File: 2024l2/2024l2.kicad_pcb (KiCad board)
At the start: 2 copper layers, 174 x 141 mm, 113 parts, among them IC1 LM2587S-ADJ, IC2 VNH5019ATR-E, IC3 VNH5019ATR-E, IC4 VNH5019ATR-E, IC5 VNH5019ATR-E, J1 Conn_01x02, J2 Conn_01x02, J3 Conn_01x03, J4 Conn_01x03, J5 Conn_01x04, J6 Conn_01x06, Q1 AON6354, Q2 AON6354, Q3 AON6354, Q4 AON6354, SW1 SW_SPDT, U1 TPS5430DDA, U2 TPS5430DDA, U3 Teensy 4.0

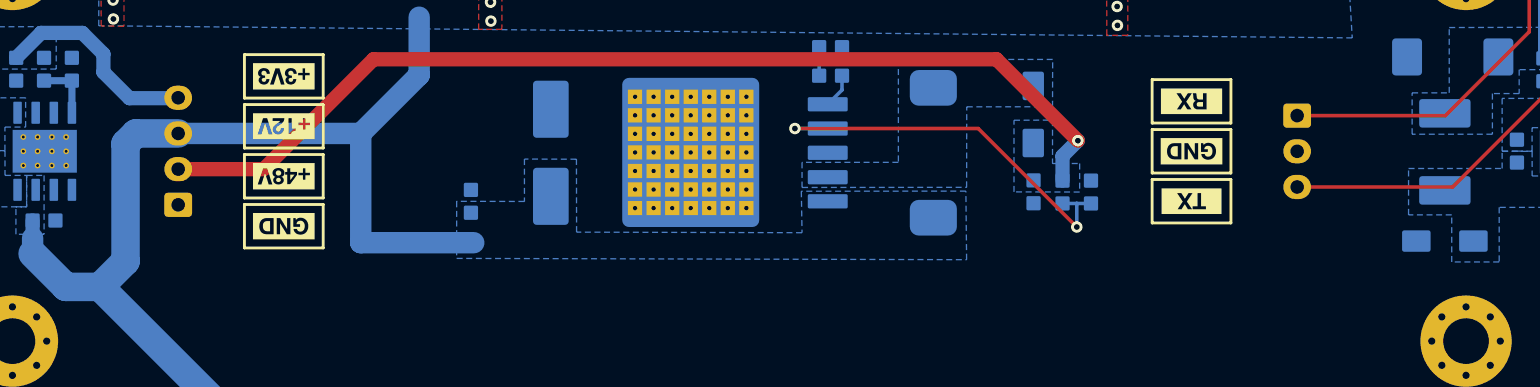
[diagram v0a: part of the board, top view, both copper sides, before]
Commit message: Minor trace adjustment
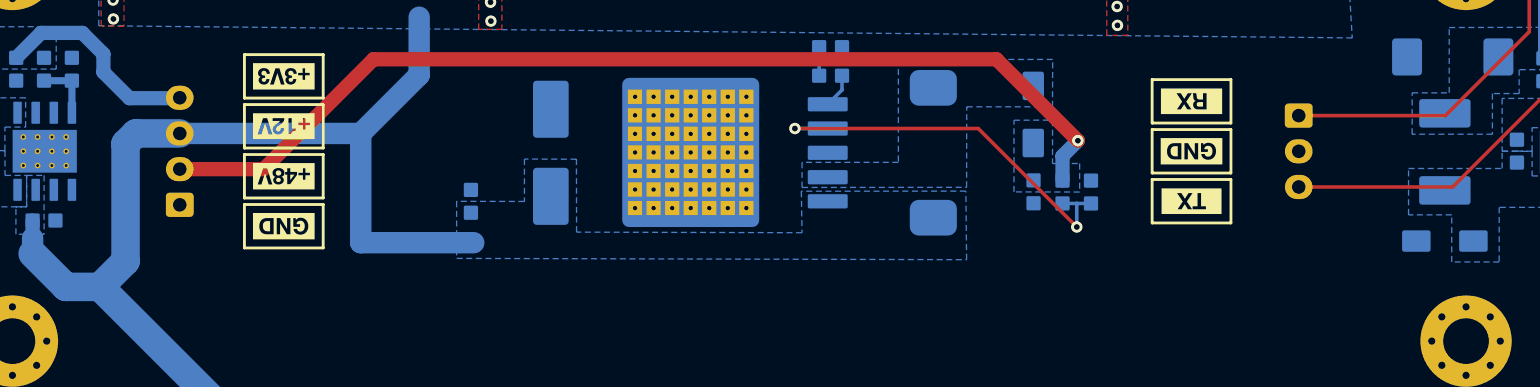
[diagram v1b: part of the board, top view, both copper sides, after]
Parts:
- moved J5 0.11 mm to (109.3, 213.6)
- moved J3 0.11 mm to (187.7, 207.4)
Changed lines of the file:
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@@
   )
   (footprint "Connector_JST:JST_XH_B4B-XH-A_1x04_P2.50mm_Vertical" (layer "B.Cu")
-    (at 109.18985 213.645 90)
+    (at 109.3 213.645 90)
     (descr "JST XH series connector, B4B-XH-A (http://www.jst-mfg.com/product/pdf/eng/eXH.pdf), generated with kicad-footprint-generator")
     (tags "connector JST XH vertical")
@@
   )
   (footprint "Connector_JST:JST_XH_B3B-XH-A_1x03_P2.50mm_Vertical" (layer "B.Cu")
-    (at 187.58985 207.395 -90)
+    (at 187.7 207.395 -90)
     (descr "JST XH series connector, B3B-XH-A (http://www.jst-mfg.com/product/pdf/eng/eXH.pdf), generated with kicad-footprint-generator")
     (tags "connector JST XH vertical")
@@
   (segment (start 124.125 151.975) (end 124.125 156.75) (width 1) (layer "F.Cu") (net 4))
   (via (at 124.125 151.975) (size 0.8) (drill 0.4) (layers "F.Cu" "B.Cu") (net 4))
+  (segment (start 99.58485 201.6) (end 102.475 201.6) (width 1) (layer "B.Cu") (net 4))
   (segment (start 124.125 139.3) (end 128.7 134.725) (width 1) (layer "B.Cu") (net 4))
+  (segment (start 92.8 183.3) (end 92.8 201.35515) (width 1) (layer "B.Cu") (net 4))
+  (segment (start 103.95 204.35) (end 105.775 206.175) (width 1) (layer "B.Cu") (net 4))
+  (segment (start 94.68985 203.245) (end 94.251637 202.806787) (width 0.25) (layer "B.Cu") (net 4))
+  (segment (start 124.125 151.975) (end 92.8 183.3) (width 1) (layer "B.Cu") (net 4))
+  (segment (start 103.95 203.075) (end 103.95 204.35) (width 1) (layer "B.Cu") (net 4))
+  (segment (start 144.6 132.025) (end 144.6 130.4) (width 1) (layer "B.Cu") (net 4))
+  (segment (start 105.775 206.175) (end 109.15985 206.175) (width 1) (layer "B.Cu") (net 4))
+  (segment (start 128.7 134.725) (end 141.9 134.725) (width 1) (layer "B.Cu") (net 4))
+  (segment (start 97.83985 203.345) (end 99.58485 201.6) (width 1) (layer "B.Cu") (net 4))
   (segment (start 102.475 201.6) (end 103.95 203.075) (width 1) (layer "B.Cu") (net 4))
-  (segment (start 103.95 203.075) (end 103.95 204.35) (width 1) (layer "B.Cu") (net 4))
-  (segment (start 105.775 206.175) (end 109.15985 206.175) (width 1) (layer "B.Cu") (net 4))
-  (segment (start 103.95 204.35) (end 105.775 206.175) (width 1) (layer "B.Cu") (net 4))
-  (segment (start 92.8 183.3) (end 92.8 201.35515) (width 1) (layer "B.Cu") (net 4))
-  (segment (start 94.68985 203.245) (end 94.251637 202.806787) (width 0.25) (layer "B.Cu") (net 4))
-  (segment (start 99.58485 201.6) (end 102.475 201.6) (width 1) (layer "B.Cu") (net 4))
-  (segment (start 97.83985 203.345) (end 99.58485 201.6) (width 1) (layer "B.Cu") (net 4))
+  (segment (start 124.125 151.975) (end 124.125 139.3) (width 1) (layer "B.Cu") (net 4))
   (segment (start 109.15985 206.175) (end 109.18985 206.145) (width 1) (layer "B.Cu") (net 4))
-  (segment (start 124.125 151.975) (end 92.8 183.3) (width 1) (layer "B.Cu") (net 4))
-  (segment (start 144.6 132.025) (end 144.6 130.4) (width 1) (layer "B.Cu") (net 4))
-  (segment (start 128.7 134.725) (end 141.9 134.725) (width 1) (layer "B.Cu") (net 4))
-  (segment (start 124.125 151.975) (end 124.125 139.3) (width 1) (layer "B.Cu") (net 4))
   (segment (start 141.9 134.725) (end 144.6 132.025) (width 1) (layer "B.Cu") (net 4))
   (segment (start 92.8 201.35515) (end 94.68985 203.245) (width 1) (layer "B.Cu") (net 4))
+  (segment (start 162.47 137.38) (end 162.47 139.67) (width 0.25) (layer "F.Cu") (net 16))
+  (segment (start 202.55 176.25) (end 202.55 181.25) (width 0.25) (layer "F.Cu") (net 16))
+  (segment (start 205.875 205) (end 198.48 212.395) (width 0.25) (layer "F.Cu") (net 16))
+  (segment (start 198.48 212.395) (end 187.7 212.395) (width 0.25) (layer "F.Cu") (net 16))
+  (segment (start 196.80559 170.50559) (end 202.55 176.25) (width 0.25) (layer "F.Cu") (net 16))
+  (segment (start 205.875 184.575) (end 205.875 205) (width 0.25) (layer "F.Cu") (net 16))
+  (segment (start 162.47 139.67) (end 193.30559 170.50559) (width 0.25) (layer "F.Cu") (net 16))
   (segment (start 193.30559 170.50559) (end 196.80559 170.50559) (width 0.25) (layer "F.Cu") (net 16))
   (segment (start 202.55 181.25) (end 205.875 184.575) (width 0.25) (layer "F.Cu") (net 16))
-  (segment (start 205.875 205) (end 198.48 212.395) (width 0.25) (layer "F.Cu") (net 16))
-  (segment (start 162.47 139.67) (end 193.30559 170.50559) (width 0.25) (layer "F.Cu") (net 16))
-  (segment (start 162.47 137.38) (end 162.47 139.67) (width 0.25) (layer "F.Cu") (net 16))
-  (segment (start 198.48 212.395) (end 187.58985 212.395) (width 0.25) (layer "F.Cu") (net 16))
-  (segment (start 196.80559 170.50559) (end 202.55 176.25) (width 0.25) (layer "F.Cu") (net 16))
-  (segment (start 202.55 176.25) (end 202.55 181.25) (width 0.25) (layer "F.Cu") (net 16))
-  (segment (start 205.875 184.575) (end 205.875 205) (width 0.25) (layer "F.Cu") (net 16))
-  (segment (start 159.93 137.38) (end 159.93 139.705) (width 0.25) (layer "F.Cu") (net 17))
+  (segment (start 159.93 139.705) (end 192.55 172.325) (width 0.25) (layer "F.Cu") (net 17))
   (segment (start 203.85 185.4) (end 203.85 201.525) (width 0.25) (layer "F.Cu") (net 17))
   (segment (start 201.825 183.375) (end 203.85 185.4) (width 0.25) (layer "F.Cu") (net 17))
+  (segment (start 203.85 201.525) (end 197.98 207.395) (width 0.25) (layer "F.Cu") (net 17))
+  (segment (start 192.55 172.325) (end 197.825 172.325) (width 0.25) (layer "F.Cu") (net 17))
+  (segment (start 201.825 176.325) (end 201.825 183.375) (width 0.25) (layer "F.Cu") (net 17))
+  (segment (start 159.93 137.38) (end 159.93 139.705) (width 0.25) (layer "F.Cu") (net 17))
   (segment (start 197.98 207.395) (end 187.58985 207.395) (width 0.25) (layer "F.Cu") (net 17))
-  (segment (start 192.55 172.325) (end 197.825 172.325) (width 0.25) (layer "F.Cu") (net 17))
-  (segment (start 159.93 139.705) (end 192.55 172.325) (width 0.25) (layer "F.Cu") (net 17))
-  (segment (start 203.85 201.525) (end 197.98 207.395) (width 0.25) (layer "F.Cu") (net 17))
   (segment (start 197.825 172.325) (end 201.825 176.325) (width 0.25) (layer "F.Cu") (net 17))
-  (segment (start 201.825 176.325) (end 201.825 183.375) (width 0.25) (layer "F.Cu") (net 17))
   (via (at 131.1 200.775) (size 0.8) (drill 0.4) (layers "F.Cu" "B.Cu") (free) (net 18))
   (via (at 104.625 199.3) (size 0.8) (drill 0.4) (layers "F.Cu" "B.Cu") (free) (net 18))
@@
   (segment (start 190.525 237.4) (end 196.5 237.4) (width 2) (layer "B.Cu") (net 18))
   (segment (start 205.925 217.480075) (end 205.925 216.269925) (width 1.5) (layer "B.Cu") (net 18))
-  (segment (start 105.5 209.35985) (end 106.21485 208.645) (width 2) (layer "B.Cu") (net 18))
+  (segment (start 105.5 217.6) (end 103.705 219.395) (width 2) (layer "B.Cu") (net 18))
   (segment (start 98.98985 217.07) (end 101.31485 219.395) (width 2) (layer "B.Cu") (net 18))
   (segment (start 201.7 237.39) (end 203.335 237.39) (width 2) (layer "B.Cu") (net 18))
   (segment (start 126.075 204.55) (end 126.075 200.5) (width 1.5) (layer "B.Cu") (net 18))
+  (segment (start 109.3 208.645) (end 106.21485 208.645) (width 2) (layer "B.Cu") (net 18))
   (segment (start 101.31485 219.395) (end 103.705 219.395) (width 2) (layer "B.Cu") (net 18))
   (segment (start 98.98985 215.97) (end 98.98985 214.745) (width 1) (layer "B.Cu") (net 18))
   (segment (start 201.69 237.4) (end 201.7 237.39) (width 2) (layer "B.Cu") (net 18))
+  (segment (start 106.21485 208.645) (end 105.5 209.35985) (width 2) (layer "B.Cu") (net 18))
+  (segment (start 105.5 209.35985) (end 105.5 217.6) (width 2) (layer "B.Cu") (net 18))
   (segment (start 103.705 219.395) (end 111.906162 227.596162) (width 2) (layer "B.Cu") (net 18))
+  (segment (start 109.3 208.645) (end 121.98 208.645) (width 1.5) (layer "B.Cu") (net 18))
   (segment (start 205.98985 214.785) (end 205.98985 216.03985) (width 1) (layer "B.Cu") (net 18))
   (segment (start 196.5 237.4) (end 201.69 237.4) (width 2) (layer "B.Cu") (net 18))
   (segment (start 121.98 208.645) (end 126.075 204.55) (width 1.5) (layer "B.Cu") (net 18))
   (segment (start 121.98 208.645) (end 121.98 216.3) (width 1.5) (layer "B.Cu") (net 18))
-  (segment (start 109.18985 208.645) (end 121.98 208.645) (width 1.5) (layer "B.Cu") (net 18))
   (segment (start 111.906162 227.596162) (end 180.721162 227.596162) (width 2) (layer "B.Cu") (net 18))
-  (segment (start 105.5 217.6) (end 105.5 209.35985) (width 2) (layer "B.Cu") (net 18))
   (segment (start 121.98 216.3) (end 129.9 216.3) (width 1.5) (layer "B.Cu") (net 18))
   (segment (start 98.98985 217.07) (end 98.98985 215.97) (width 1.5) (layer "B.Cu") (net 18))
   (segment (start 180.721162 227.596162) (end 190.525 237.4) (width 2) (layer "B.Cu") (net 18))
-  (segment (start 103.705 219.395) (end 105.5 217.6) (width 2) (layer "B.Cu") (net 18))
   (segment (start 206.025 234.7) (end 206.025 217.48515) (width 2) (layer "B.Cu") (net 18))
   (segment (start 203.335 237.39) (end 206.025 234.7) (width 2) (layer "B.Cu") (net 18))
-  (segment (start 106.21485 208.645) (end 109.18985 208.645) (width 2) (layer "B.Cu") (net 18))
+  (segment (start 166.525 203.45) (end 122.875 203.45) (width 1) (layer "F.Cu") (net 23))
+  (segment (start 115.18 211.145) (end 109.3 211.145) (width 1) (layer "F.Cu") (net 23))
   (segment (start 172.225 209.15) (end 166.525 203.45) (width 1) (layer "F.Cu") (net 23))
-  (segment (start 115.18 211.145) (end 109.18985 211.145) (width 1) (layer "F.Cu") (net 23))
   (segment (start 122.875 203.45) (end 115.18 211.145) (width 1) (layer "F.Cu") (net 23))
-  (segment (start 166.525 203.45) (end 122.875 203.45) (width 1) (layer "F.Cu") (net 23))
   (via (at 172.225 209.15) (size 0.8) (drill 0.4) (layers "F.Cu" "B.Cu") (net 23))
   (segment (start 171.15 211.95) (end 171.15 210.225) (width 1) (layer "B.Cu") (net 23))
